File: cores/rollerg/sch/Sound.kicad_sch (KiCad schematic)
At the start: 31 parts, among them J1 XTAL_OSC

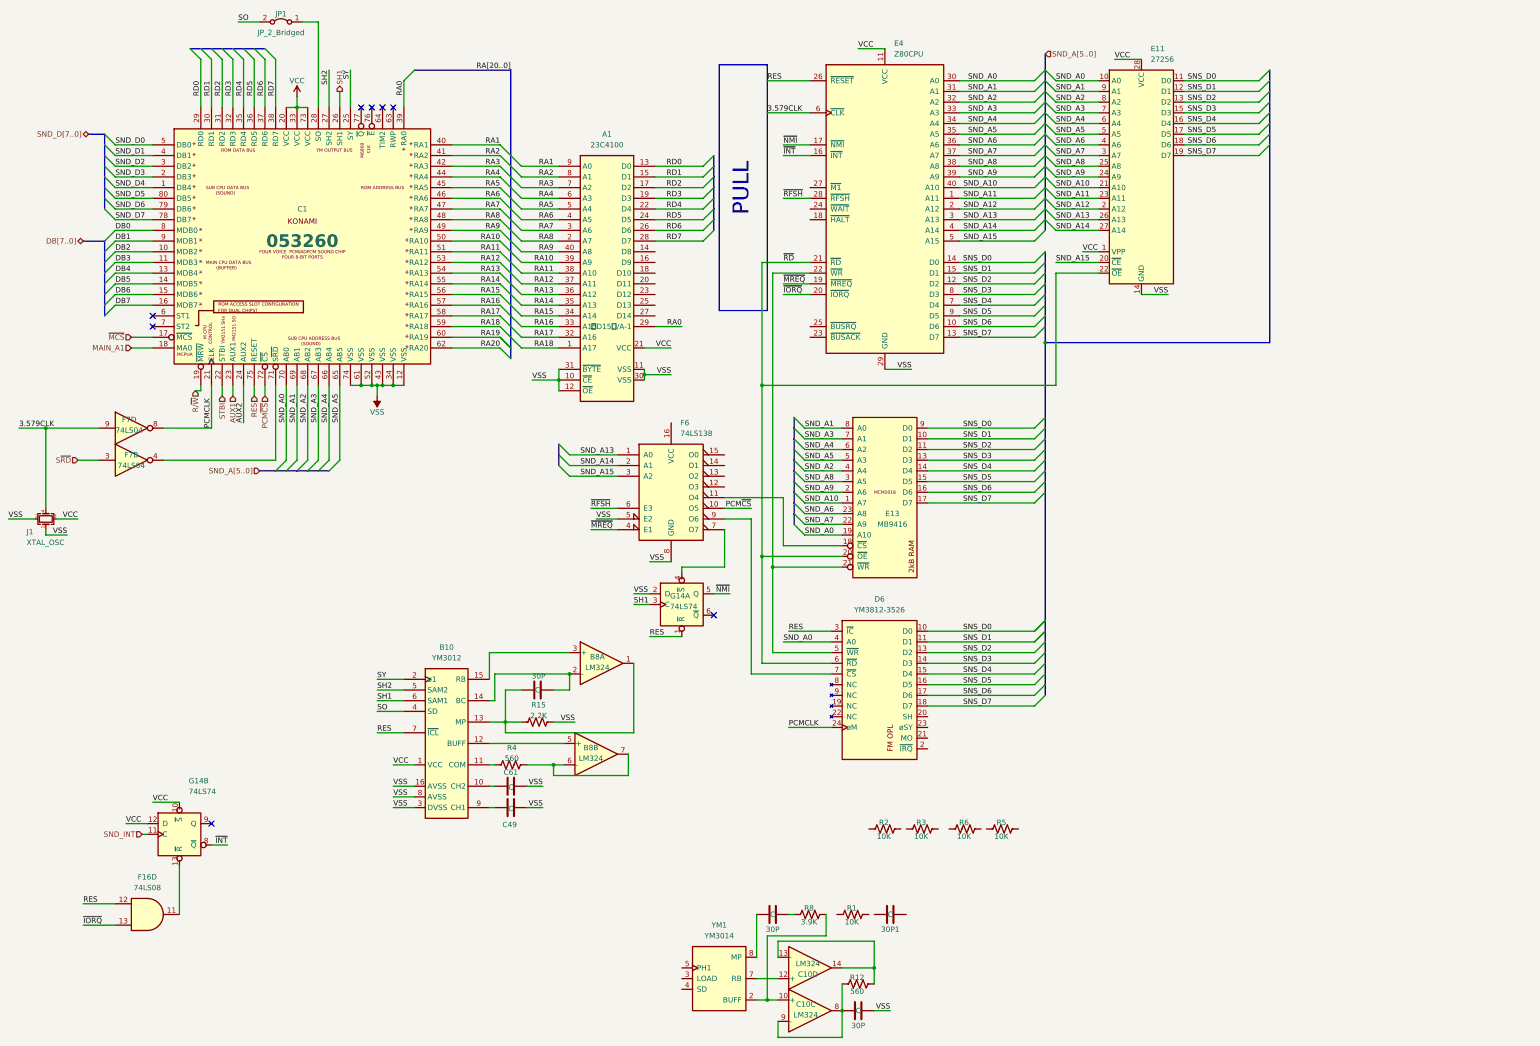
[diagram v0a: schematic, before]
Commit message: almost complete rollerg sch
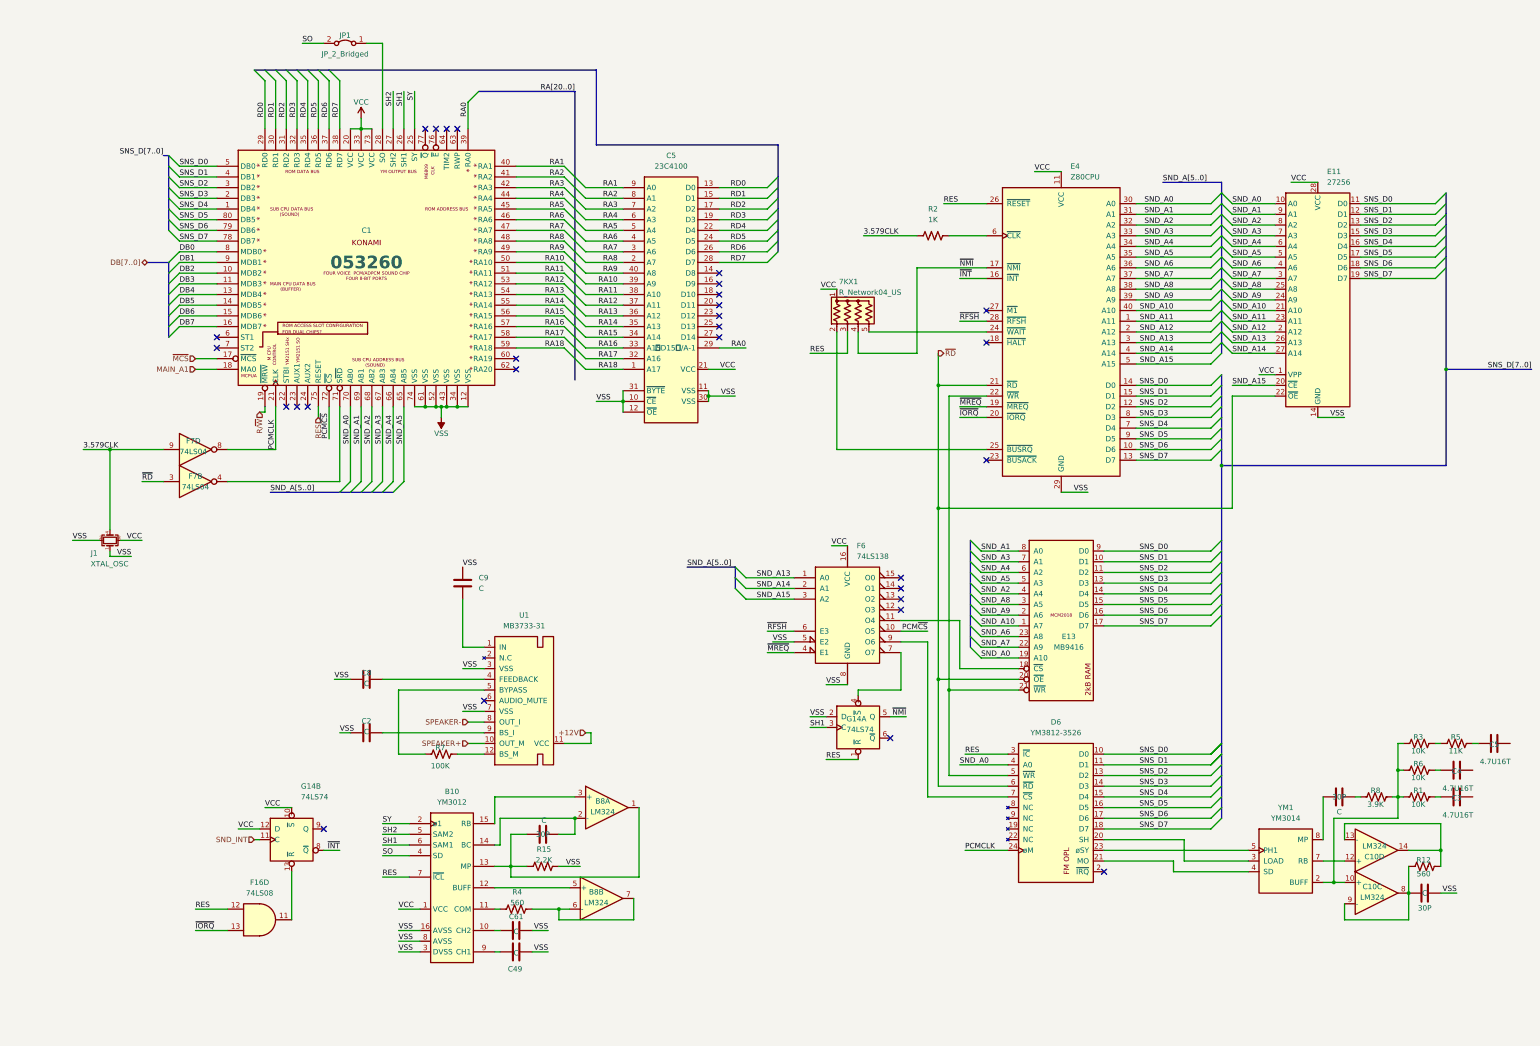
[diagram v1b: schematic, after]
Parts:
- removed 30P1: C, symbol Device:C
- added 7KX1: R_Network04_US, Resistor_THT:R_Array_SIP5, symbol Device:R_Network04_US
- added C2, C8, C9: C, symbol Device:C
- added C3, C4, C5: 4.7U16T, symbol Device:C
- added R7: 100K, symbol Device:R_US
- added U1: MB3733-31, symbol arcade:MB3733-31
- C: renamed from 30P; value C -> 30P
- R2: value 10K -> 1K
- R5: value 10K -> 11K
- renumbered A1 to C5
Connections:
- net SND_D0 is gone; now on net SNS_D0: C1.5 (DB0)
- net SND_D1 is gone; now on net SNS_D1: C1.4 (DB1)
- net SND_D2 is gone; now on net SNS_D2: C1.3 (DB2)
- net SND_D3 is gone; now on net SNS_D3: C1.2 (DB3)
- net SND_D4 is gone; now on net SNS_D4: C1.1 (DB4)
- net SND_D5 is gone; now on net SNS_D5: C1.80 (DB5)
- net SND_D6 is gone; now on net SNS_D6: C1.79 (DB6)
- net SND_D7 is gone; now on net SNS_D7: C1.78 (DB7)
- net S~{RD} is gone; now on net ~{RD}: F7.3
- net 3.579CLK: now also R2.1; no longer E4.6 (~{CLK})
- net RES: now also 7KX1.3 (R2)
- net VCC: now also F6.16 (VCC), 7KX1.1 (common)
- net VSS: now also C2.2, C8.2, C9.1, U1.3 (VSS), U1.7 (VSS)
- net ~{NMI}: now also 7KX1.4 (R3)
- net at R1.1: now also C10.10 (+), R3.1, R6.1, R8.2, YM1.2 (BUFF)
- net at R1.2: now also C3.1
- net at E4.24 (~{WAIT}): now also 7KX1.5 (R4)
- net at E4.25 (~{BUSRQ}): now also 7KX1.2 (R1)
- net at D6.20 (SH): now also YM1.3 (LOAD)
- net at D6.21 (MO): now also YM1.4 (SD)
- net at D6.23 (øSY): now also YM1.5 (PH1)
- net at R3.2: now also R5.1
- net at R2.2: now also E4.6 (~{CLK})
- net at R6.2: now also C4.1
- net at R5.2: now also C5.1
- net AUX1: no longer names the net of C1.23 (AUX1)
- net AUX2: no longer names the net of C1.24 (AUX2)
- net RA19: no longer names the net of C1.60 (RA19)
- net RA20: no longer names the net of C1.62 (RA20)
- net STBI: no longer names the net of C1.22 (STBI)
- new net: C2.1, U1.9 (BS_I)
- new net: C9.2, U1.1 (IN)
- new net: C8.1, U1.4 (FEEDBACK)
- new net: R7.2, U1.12 (BS_M)
- new net: R7.1, U1.5 (BYPASS)
- new net +12V: U1.11 (VCC)
- new net SPEAKER+: U1.10 (OUT_M)
- new net SPEAKER-: U1.8 (OUT_I)
- no-connect marks 8 -> 29
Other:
- moved on the sheet: 30P, B10, B8A, B8B, C, C1, C10C, C10D, C49, C5, C61, D6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
